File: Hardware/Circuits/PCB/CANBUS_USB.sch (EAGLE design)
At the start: 33 parts

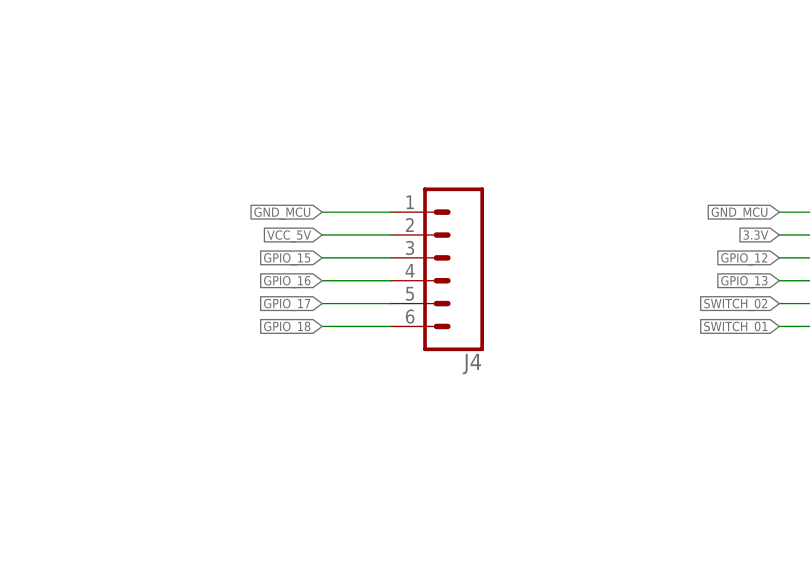
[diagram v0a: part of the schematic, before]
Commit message: circuits
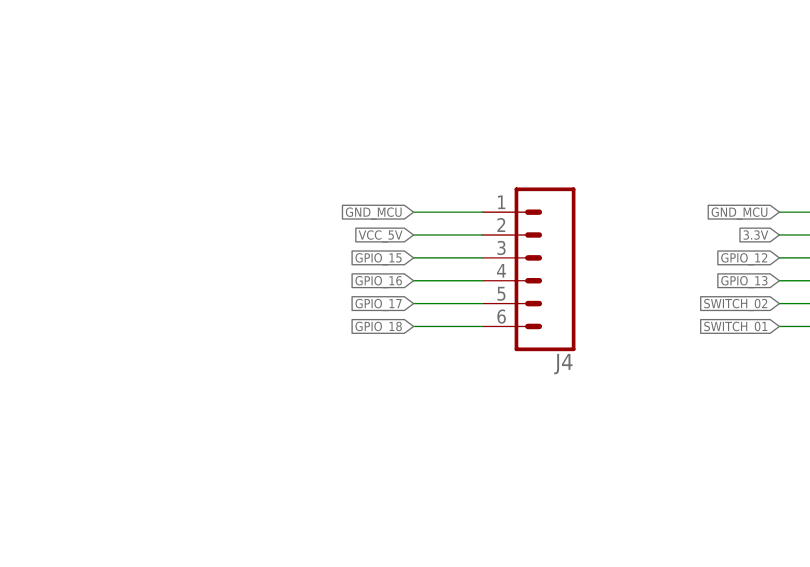
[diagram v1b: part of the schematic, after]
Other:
- moved on the sheet: J4
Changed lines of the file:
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@@
 <?xml version="1.0" encoding="utf-8"?>
 <!DOCTYPE eagle SYSTEM "eagle.dtd">
-<eagle version="9.5.2">
+<eagle version="9.6.2">
 <drawing>
 <settings>
@@
 <attribute name="VALUE" x="364.49" y="155.702" size="1.778" layer="96" rot="R180"/>
 </instance>
-<instance part="J4" gate="G$1" x="223.52" y="144.78" smashed="yes" rot="R180">
-<attribute name="VALUE" x="228.6" y="154.686" size="1.778" layer="96" font="vector" rot="R180"/>
-<attribute name="NAME" x="228.6" y="134.112" size="1.778" layer="95" font="vector" rot="R180"/>
+<instance part="J4" gate="G$1" x="233.68" y="144.78" smashed="yes" rot="R180">
+<attribute name="VALUE" x="238.76" y="154.686" size="1.778" layer="96" font="vector" rot="R180"/>
+<attribute name="NAME" x="238.76" y="134.112" size="1.778" layer="95" font="vector" rot="R180"/>
 </instance>
 </instances>
@@
 <segment>
 <pinref part="J4" gate="G$1" pin="1"/>
-<wire x1="218.44" y1="149.86" x2="210.82" y2="149.86" width="0.1524" layer="91"/>
-<label x="210.82" y="149.86" size="1.016" layer="95" rot="R180" xref="yes"/>
+<wire x1="228.6" y1="149.86" x2="220.98" y2="149.86" width="0.1524" layer="91"/>
+<label x="220.98" y="149.86" size="1.016" layer="95" rot="R180" xref="yes"/>
 </segment>
 </net>
@@
 <segment>
 <pinref part="J4" gate="G$1" pin="4"/>
-<wire x1="218.44" y1="142.24" x2="210.82" y2="142.24" width="0.1524" layer="91"/>
-<label x="210.82" y="142.24" size="1.016" layer="95" rot="R180" xref="yes"/>
+<wire x1="228.6" y1="142.24" x2="220.98" y2="142.24" width="0.1524" layer="91"/>
+<label x="220.98" y="142.24" size="1.016" layer="95" rot="R180" xref="yes"/>
 </segment>
 </net>
@@
 <segment>
 <pinref part="J4" gate="G$1" pin="5"/>
-<wire x1="218.44" y1="139.7" x2="210.82" y2="139.7" width="0.1524" layer="91"/>
-<label x="210.82" y="139.7" size="1.016" layer="95" rot="R180" xref="yes"/>
+<wire x1="228.6" y1="139.7" x2="220.98" y2="139.7" width="0.1524" layer="91"/>
+<label x="220.98" y="139.7" size="1.016" layer="95" rot="R180" xref="yes"/>
 </segment>
 </net>
@@
 <segment>
 <pinref part="J4" gate="G$1" pin="6"/>
-<wire x1="218.44" y1="137.16" x2="210.82" y2="137.16" width="0.1524" layer="91"/>
-<label x="210.82" y="137.16" size="1.016" layer="95" rot="R180" xref="yes"/>
+<wire x1="228.6" y1="137.16" x2="220.98" y2="137.16" width="0.1524" layer="91"/>
+<label x="220.98" y="137.16" size="1.016" layer="95" rot="R180" xref="yes"/>
 </segment>
 </net>
@@
 <segment>
 <pinref part="J4" gate="G$1" pin="2"/>
-<wire x1="218.44" y1="147.32" x2="210.82" y2="147.32" width="0.1524" layer="91"/>
-<label x="210.82" y="147.32" size="1.016" layer="95" rot="R180" xref="yes"/>
+<wire x1="228.6" y1="147.32" x2="220.98" y2="147.32" width="0.1524" layer="91"/>
+<label x="220.98" y="147.32" size="1.016" layer="95" rot="R180" xref="yes"/>
 </segment>
 </net>
@@
 <segment>
 <pinref part="J4" gate="G$1" pin="3"/>
-<wire x1="218.44" y1="144.78" x2="210.82" y2="144.78" width="0.1524" layer="91"/>
-<label x="210.82" y="144.78" size="1.016" layer="95" rot="R180" xref="yes"/>
-</segment>
-</net>
+<wire x1="228.6" y1="144.78" x2="220.98" y2="144.78" width="0.1524" layer="91"/>
+<label x="220.98" y="144.78" size="1.016" layer="95" rot="R180" xref="yes"/>
+</segment>
+</net>
